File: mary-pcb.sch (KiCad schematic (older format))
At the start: 18 parts

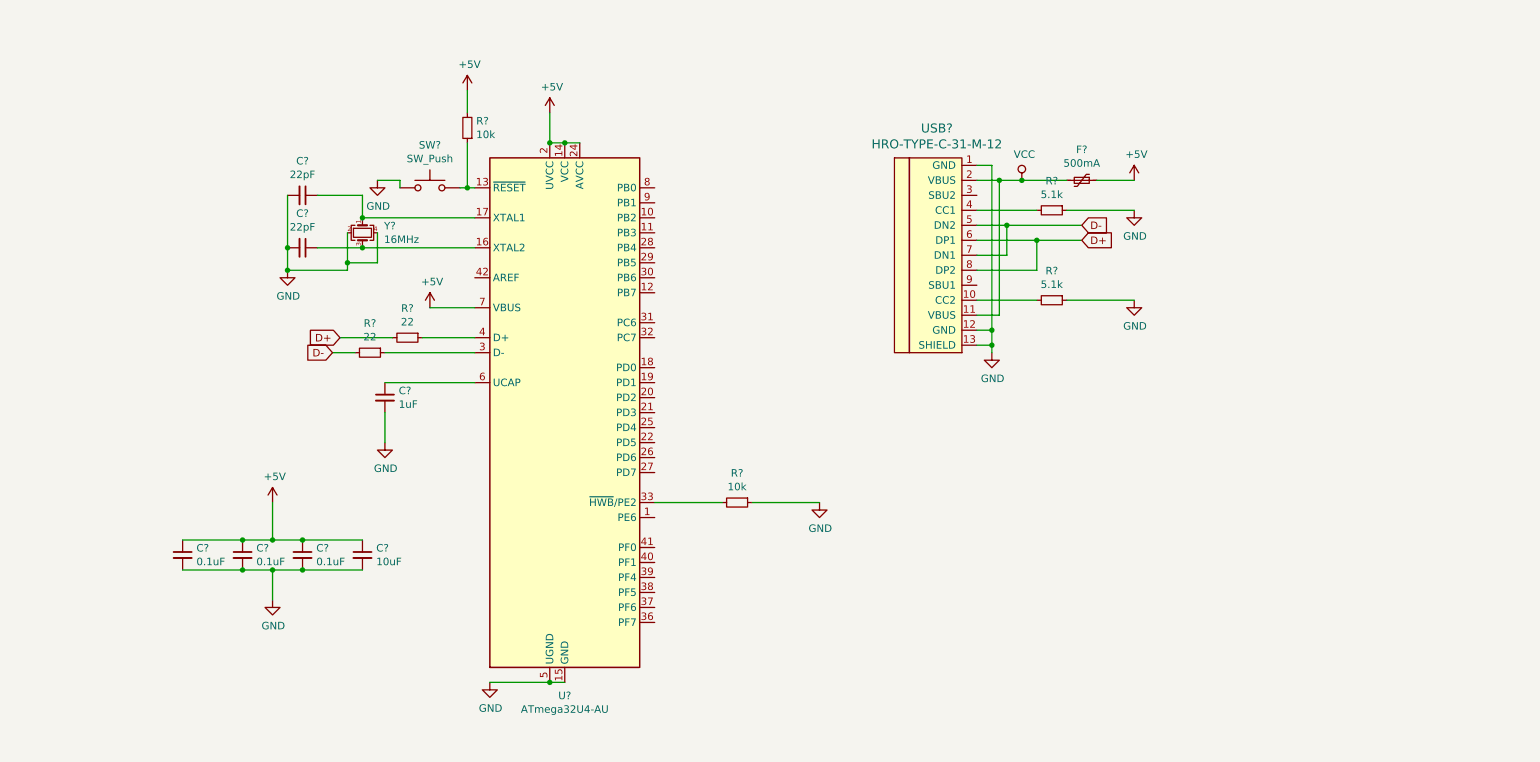
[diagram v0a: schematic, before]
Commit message: complete keyboard matrix
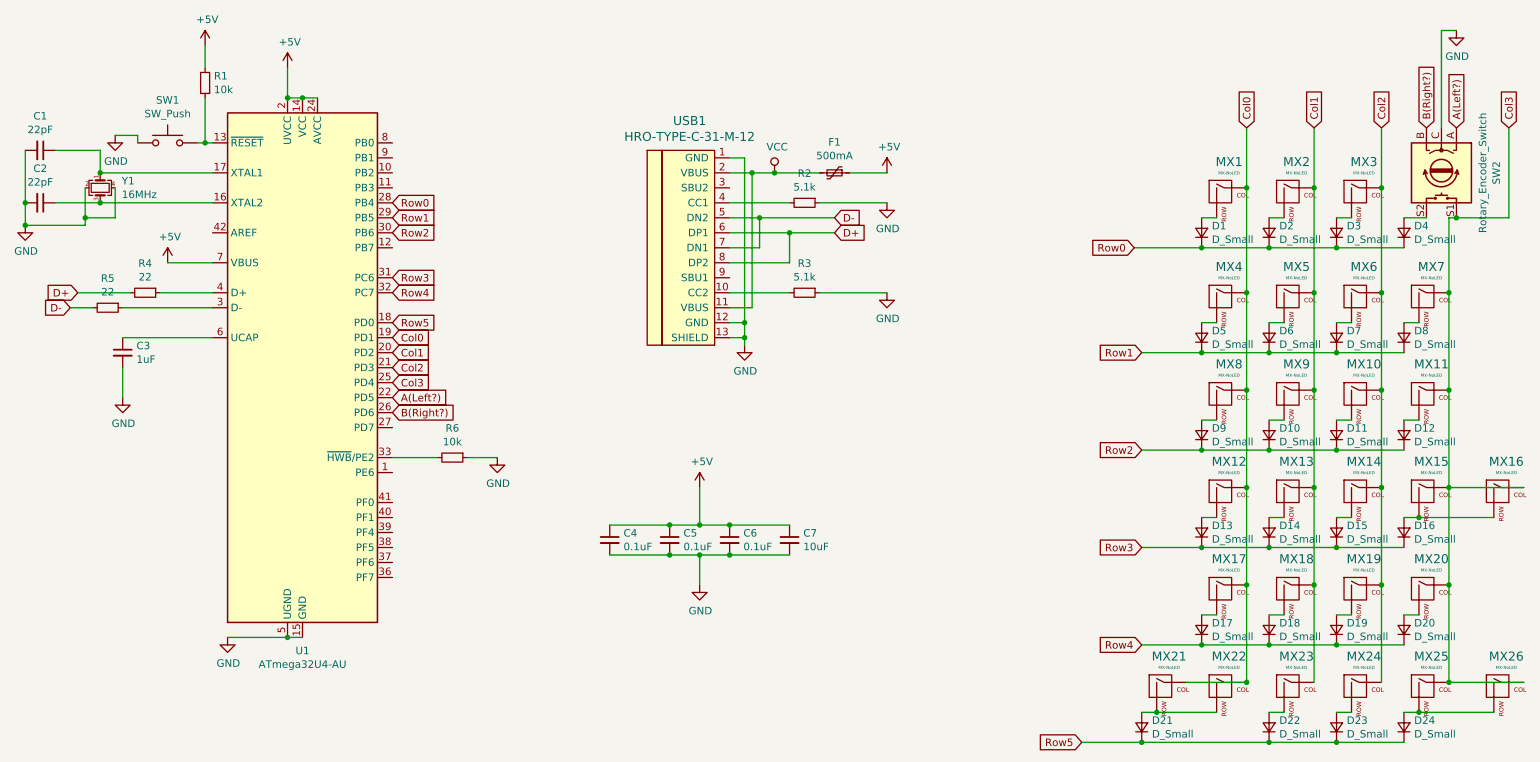
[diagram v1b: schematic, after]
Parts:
- added D1, D10, D11, D12, D13, D14, D15, D16, D17, D18, D19, D2, D20, D21, D22, D23, D24, D3, D4, D5, D6, D7, D8, D9: D_Small, symbol Device:D_Small
- added MX1, MX10, MX11, MX12, MX13, MX14, MX15, MX16, MX17, MX18, MX19, MX2, MX20, MX21, MX22, MX23, MX24, MX25, MX26, MX3, MX4, MX5, MX6, MX7, MX8, MX9: MX-NoLED, symbol MX_Alps_Hybrid:MX-NoLED
- added SW2: Rotary_Encoder_Switch, symbol Device:Rotary_Encoder_Switch
- gave numbers to parts that had none: 18
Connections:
- net GND: now also SW2.C
- net Row5: now reaches U1.18 (PD0)
- net Row5: now also D21.1 (K), D22.1 (K), D23.1 (K), D24.1 (K)
- net Col0: now reaches U1.19 (PD1)
- net Col0: now also MX1.1 (COL), MX12.1 (COL), MX17.1 (COL), MX21.1 (COL), MX22.1 (COL), MX4.1 (COL), MX8.1 (COL)
- net Col1: now reaches U1.20 (PD2)
- net Col1: now also MX13.1 (COL), MX18.1 (COL), MX2.1 (COL), MX23.1 (COL), MX5.1 (COL), MX9.1 (COL)
- net Col2: now reaches U1.21 (PD3)
- net Col2: now also MX10.1 (COL), MX14.1 (COL), MX19.1 (COL), MX24.1 (COL), MX3.1 (COL), MX6.1 (COL)
- net A(Left?): now reaches U1.22 (PD5)
- net A(Left?): now also SW2.A
- net Col3: now reaches U1.25 (PD4)
- net Col3: now also MX11.1 (COL), MX15.1 (COL), MX16.1 (COL), MX20.1 (COL), MX25.1 (COL), MX26.1 (COL), MX7.1 (COL), SW2.S1
- net B(Right?): now reaches U1.26 (PD6)
- net B(Right?): now also SW2.B
- net Row0: now reaches U1.28 (PB4)
- net Row0: now also D1.1 (K), D2.1 (K), D3.1 (K), D4.1 (K)
- net Row1: now reaches U1.29 (PB5)
- net Row1: now also D5.1 (K), D6.1 (K), D7.1 (K), D8.1 (K)
- net Row2: now reaches U1.30 (PB6)
- net Row2: now also D10.1 (K), D11.1 (K), D12.1 (K), D9.1 (K)
- net Row3: now reaches U1.31 (PC6)
- net Row3: now also D13.1 (K), D14.1 (K), D15.1 (K), D16.1 (K)
- net Row4: now reaches U1.32 (PC7)
- net Row4: now also D17.1 (K), D18.1 (K), D19.1 (K), D20.1 (K)
- new net: D1.2 (A), MX1.2 (ROW)
- new net: D2.2 (A), MX2.2 (ROW)
- new net: D3.2 (A), MX3.2 (ROW)
- new net: D5.2 (A), MX4.2 (ROW)
- new net: D6.2 (A), MX5.2 (ROW)
- new net: D7.2 (A), MX6.2 (ROW)
- new net: D8.2 (A), MX7.2 (ROW)
- new net: D9.2 (A), MX8.2 (ROW)
- new net: D10.2 (A), MX9.2 (ROW)
- new net: D11.2 (A), MX10.2 (ROW)
- new net: D13.2 (A), MX12.2 (ROW)
- new net: D14.2 (A), MX13.2 (ROW)
- new net: D15.2 (A), MX14.2 (ROW)
- new net: D17.2 (A), MX17.2 (ROW)
- new net: D18.2 (A), MX18.2 (ROW)
- new net: D19.2 (A), MX19.2 (ROW)
- new net: D21.2 (A), MX21.2 (ROW), MX22.2 (ROW)
- new net: D23.2 (A), MX24.2 (ROW)
- new net: D20.2 (A), MX20.2 (ROW)
- new net: D22.2 (A), MX23.2 (ROW)
- new net: D12.2 (A), MX11.2 (ROW)
- new net: D16.2 (A), MX15.2 (ROW), MX16.2 (ROW)
- new net: D24.2 (A), MX25.2 (ROW), MX26.2 (ROW)
- new net: D4.2 (A), SW2.S2
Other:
- moved on the sheet: C1, C2, C3, C4, C5, C6, C7, F1, R1, R2, R3, R4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

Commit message: assign footprints
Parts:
- C1, C2, C3, C4, C5, C6, C7: footprint (none) -> Capacitor_SMD:C_0805_2012Metric
- D1, D10, D11, D12, D13, D14, D15, D16, D17, D18, D19, D2, D20, D21, D22, D23, D24, D3, D4, D5, D6, D7, D8, D9: footprint (none) -> Diode_SMD:D_SOD-123
- F1: footprint (none) -> Fuse:Fuse_1206_3216Metric
- MX1, MX10, MX11, MX12, MX13, MX14, MX15, MX17, MX18, MX19, MX2, MX20, MX22, MX23, MX24, MX25, MX3, MX4, MX5, MX6, MX7, MX8, MX9: footprint (none) -> MX_Alps_Hybrid:MX-1U-NoLED
- MX16, MX21, MX26: footprint (none) -> MX_Alps_Hybrid:MX-2U-ReversedStabilizers-NoLED
- R1, R2, R3, R4, R5, R6: footprint (none) -> Resistor_SMD:R_0805_2012Metric
- SW1: footprint (none) -> random-keyboard-parts:SKQG-1155865
- SW2: footprint (none) -> Keebio-Parts:RotaryEncoder_EC11
- USB1: footprint (none) -> Type-C:HRO-TYPE-C-31-M-12
- Y1: footprint (none) -> Crystal:Crystal_SMD_3225-4Pin_3.2x2.5mm
